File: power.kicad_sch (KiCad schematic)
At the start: 6 parts, among them U19 SN74ALS04 (КР1533ЛН1), U21 SN74ALS14 (КР1533ТЛ2), U39 IN74ALS32N (КР1533ЛЛ1), U40 IN74ALS00N (КР1533ЛА3), U75 IN74ALS32N (КР1533ЛЛ1)

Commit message: March 26th update
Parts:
- U19, U21, U39, U40, U75: footprint Package_DIP:DIP-14_W7.62mm_Socket_LongPads -> Package_DIP:DIP-14_W7.62mm_Socket
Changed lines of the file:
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@@
       (effects (font (size 1.27 1.27)) (justify left))
     )
-    (property "Footprint" "Package_DIP:DIP-14_W7.62mm_Socket_LongPads" (id 2) (at 54.61 41.91 0)
+    (property "Footprint" "Package_DIP:DIP-14_W7.62mm_Socket" (id 2) (at 54.61 41.91 0)
       (effects (font (size 1.27 1.27)) hide)
     )
@@
       (effects (font (size 1.27 1.27)) (justify left))
     )
-    (property "Footprint" "Package_DIP:DIP-14_W7.62mm_Socket_LongPads" (id 2) (at 107.95 41.91 0)
+    (property "Footprint" "Package_DIP:DIP-14_W7.62mm_Socket" (id 2) (at 107.95 41.91 0)
       (effects (font (size 1.27 1.27)) hide)
     )
@@
       (effects (font (size 1.27 1.27)) (justify left))
     )
-    (property "Footprint" "Package_DIP:DIP-14_W7.62mm_Socket_LongPads" (id 2) (at 37.465 41.91 0)
+    (property "Footprint" "Package_DIP:DIP-14_W7.62mm_Socket" (id 2) (at 37.465 41.91 0)
       (effects (font (size 1.27 1.27)) hide)
     )
@@
       (effects (font (size 1.27 1.27)) (justify left))
     )
-    (property "Footprint" "Package_DIP:DIP-14_W7.62mm_Socket_LongPads" (id 2) (at 89.535 41.91 0)
+    (property "Footprint" "Package_DIP:DIP-14_W7.62mm_Socket" (id 2) (at 89.535 41.91 0)
       (effects (font (size 1.27 1.27)) hide)
     )
@@
       (effects (font (size 1.27 1.27)) (justify left))
     )
-    (property "Footprint" "Package_DIP:DIP-14_W7.62mm_Socket_LongPads" (id 2) (at 72.39 41.91 0)
+    (property "Footprint" "Package_DIP:DIP-14_W7.62mm_Socket" (id 2) (at 72.39 41.91 0)
       (effects (font (size 1.27 1.27)) hide)
     )

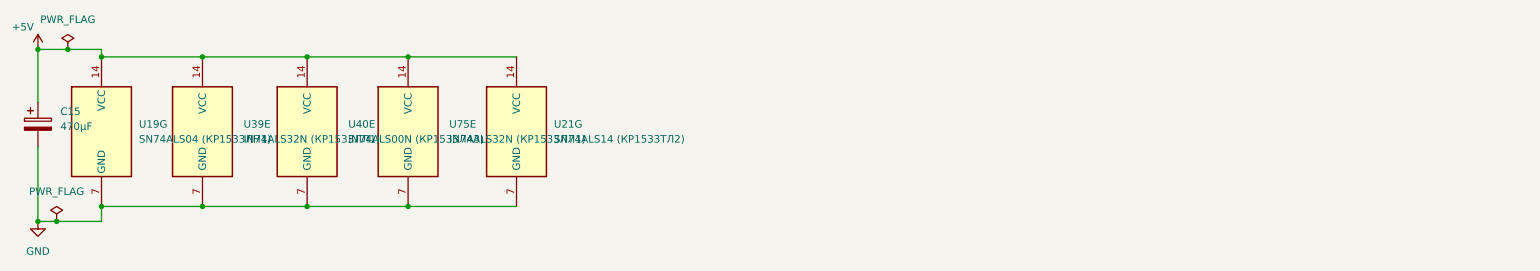
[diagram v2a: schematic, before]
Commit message: March 31st Update
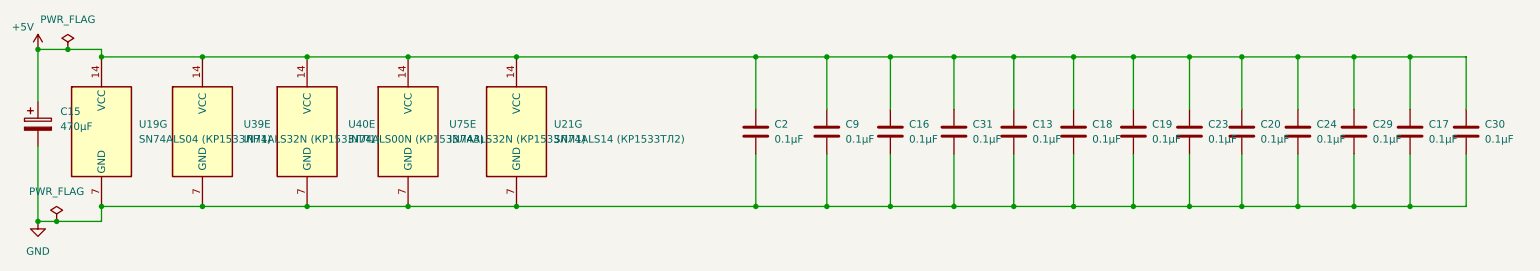
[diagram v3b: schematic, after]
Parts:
- added C13, C16, C17, C18, C19, C2, C20, C23, C24, C29, C30, C31, C9: 0.1μF, Capacitor_THT:C_Disc_D7.0mm_W2.5mm_P5.00mm, symbol Device:C
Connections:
- net +5V: now also C13.1, C16.1, C17.1, C18.1, C19.1, C2.1, C20.1, C23.1, C24.1, C29.1, C30.1, C31.1, C9.1
- net GND: now also C13.2, C16.2, C17.2, C18.2, C19.2, C2.2, C20.2, C23.2, C24.2, C29.2, C30.2, C31.2, C9.2
